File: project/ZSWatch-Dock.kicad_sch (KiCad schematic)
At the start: 34 parts, among them IC1 XC9265C181MR-G, IC2 MIC5219-3.3YM5, IC3 NTS0104GU12, IC4 STM32F072CBT6, Q1 BSH205G2AR, SW2 CHARGE, X1 WATCH, X3 DEBUG, X4 USB4105-GF-A

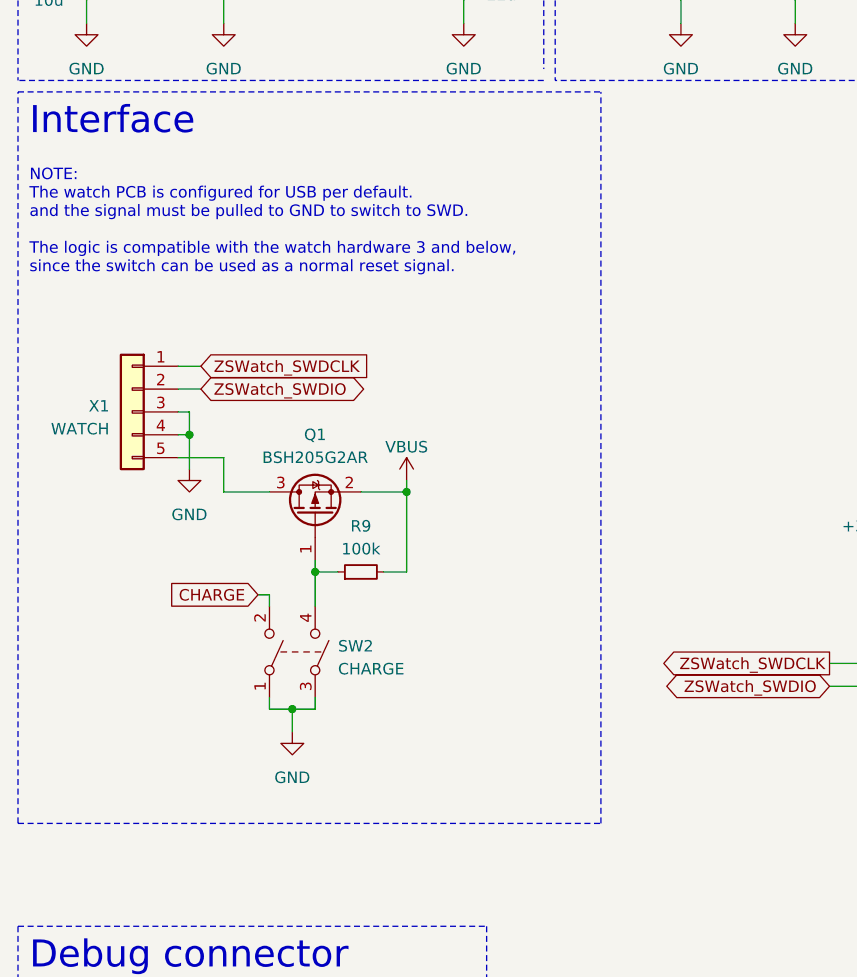
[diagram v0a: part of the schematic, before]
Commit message: fixup! - Add QR code with link to GitHub repository - Add switch to enable / disable charging - Remove reset line from STM32 to the watch connector
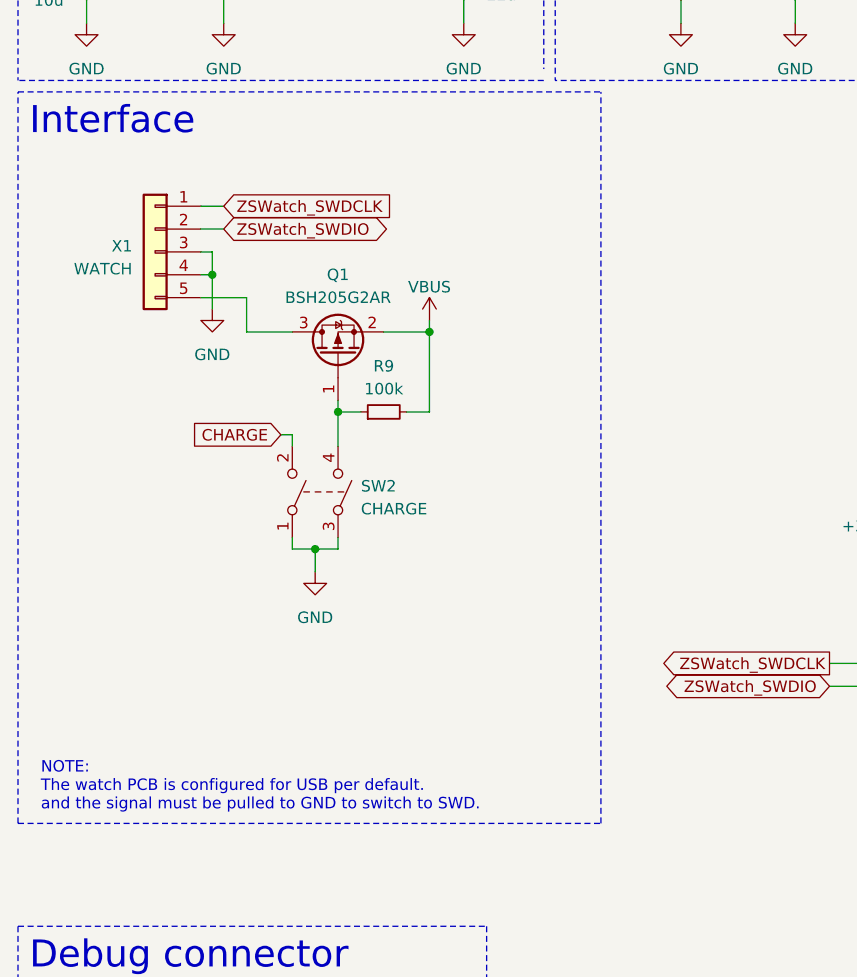
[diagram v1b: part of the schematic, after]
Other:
- note added: "NOTE: The watch PCB is configured for USB per default. and the signal must be pulled to GND to switch to SWD."
- note removed: "NOTE: The watch PCB is configured for USB per default. and the signal must be pulled to GND to switch to SWD. The logic is compatible with the watch hardware 3 and below, since the switch can be used as a normal reset signal."
- moved on the sheet: Q1, R9, SW2, X1
